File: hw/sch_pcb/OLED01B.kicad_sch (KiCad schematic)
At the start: 33 parts, among them J1 HEADER_2x03_PARALLEL, J2 HEADER_2x04_PARALLEL, J3 HEADER_1x03, J4 HEADER_2x05_PARALLEL, U1 MAX5026

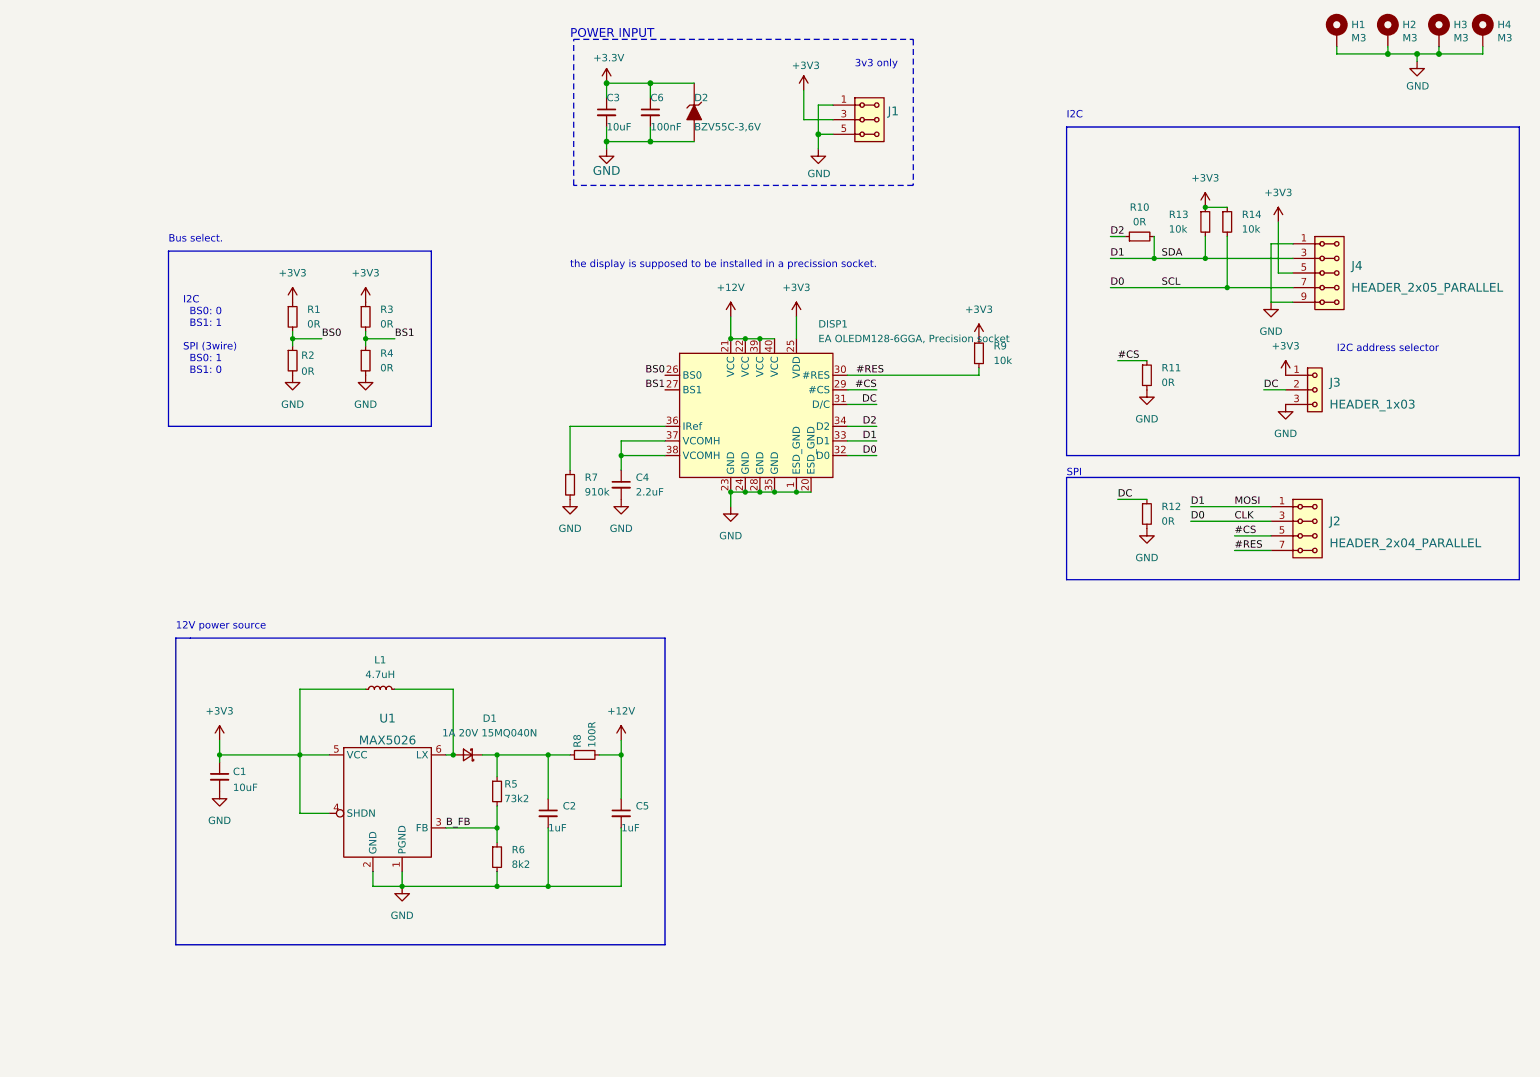
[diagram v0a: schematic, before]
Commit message: Update schematics
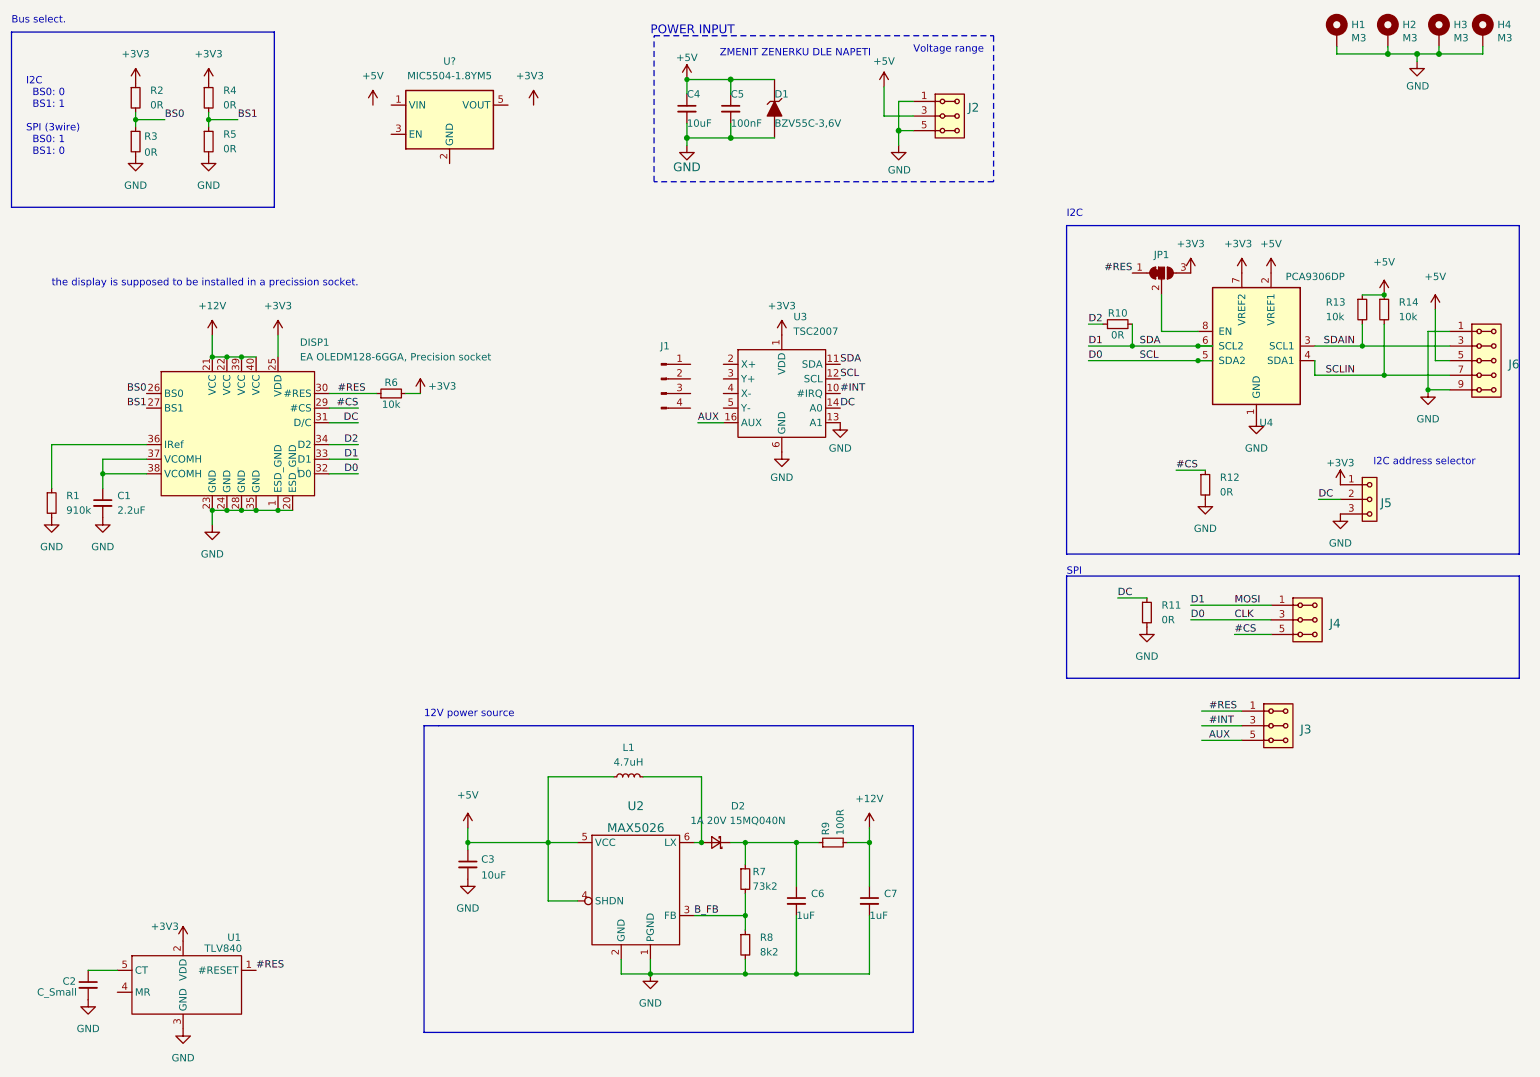
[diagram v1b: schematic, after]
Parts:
- added C2: C_Small, symbol Device:C_Small
- added J1: Conn_01x04_Male, Connector_FFC-FPC:TE_84952-4_1x04-1MP_P1.0mm_Horizontal, symbol Connector:Conn_01x04_Male
- added J3: HEADER_2x03_PARALLEL, symbol MLAB_HEADER:HEADER_2x03_PARALLEL
- added JP1: SolderJumper_3_Bridged12, symbol Jumper:SolderJumper_3_Bridged12
- added U1: TLV840, Package_TO_SOT_SMD:SOT-23-5, symbol MLAB_IO:TLV840
- added U3: TSC2007, Package_SO:TSSOP-16_4.4x5mm_P0.65mm, symbol MLAB_IO:TSC2007
- added U4: PCA9306DP, Package_SO:TSSOP-8_3x3mm_P0.65mm, symbol Interface:PCA9306DP
- added U?: MIC5504-1.8YM5, Package_TO_SOT_SMD:SOT-23-5, symbol Regulator_Linear:MIC5504-1.8YM5
- D1: renamed from D2; UST_ID 5c70984512875079b91f88b1 -> (none)
- J4: renamed from J2; value HEADER_2x04_PARALLEL -> HEADER_2x03_PARALLEL; footprint Mlab_Pin_Headers:Straight_2x04 -> Mlab_Pin_Headers:Straight_2x03; symbol MLAB_HEADER:HEADER_2x04_PARALLEL -> MLAB_HEADER:HEADER_2x03_PARALLEL
- renumbered C4 to C1, C1 to C3, C3 to C4, C6 to C5, C2 to C6, C5 to C7, D1 to D2, J1 to J2, J3 to J5, J4 to J6, R7 to R1, R12 to R11, R11 to R12, R1 to R2, R2 to R3, R3 to R4, R4 to R5, R9 to R6, R5 to R7, R6 to R8, R8 to R9, U1 to U2
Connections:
- net #RES: now also R6.1, J3.1, J3.2, JP1.1 (A), U1.1 (#RESET); no longer J4.7, J4.8, R6.2
- net +3V3: now also R6.2, JP1.3 (B), U1.2 (VDD), U3.1 (VDD), U4.7 (VREF2); no longer C3.1, C4.1, C5.1, D1.1 (K), J2.3, J2.4, J6.5, J6.6, L1.1, R13.1, R14.1, R6.1, U2.4 (SHDN), U2.5 (VCC)
- net CLK: now also U3.12 (SCL), U4.5 (SDA2); no longer J6.7, J6.8, R14.2
- net D1: now also U3.11 (SDA), U4.6 (SCL2); no longer J6.3, J6.4, R13.2
- net DC: now also U3.14 (A0)
- net GND: now also C2.2, U1.3 (GND), U3.13 (A1), U3.6 (GND), U4.1 (GND)
- new net: JP1.2 (C), U4.8 (EN)
- new net: C2.1, U1.5 (CT)
- new net #INT: J3.3, J3.4, U3.10 (#IRQ)
- new net +5V: C3.1, C4.1, C5.1, D1.1 (K), J2.3, J2.4, J6.5, J6.6, L1.1, R13.1, R14.1, U2.4 (SHDN), U2.5 (VCC), U4.2 (VREF1)
- new net AUX: J3.5, J3.6, U3.16 (AUX)
- new net SCLIN: J6.7, J6.8, R14.2, U4.4 (SDA1)
- new net SDAIN: J6.3, J6.4, R13.2, U4.3 (SCL1)
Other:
- note added: "Voltage range"
- note added: "ZMENIT ZENERKU DLE NAPETI"
- note removed: "3v3 only"
- moved on the sheet: C1, C3, C4, C5, C6, C7, D1, D2, DISP1, J2, J5, J6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
